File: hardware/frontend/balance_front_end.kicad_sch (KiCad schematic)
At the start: 5 parts, among them Q601 BSS308PE

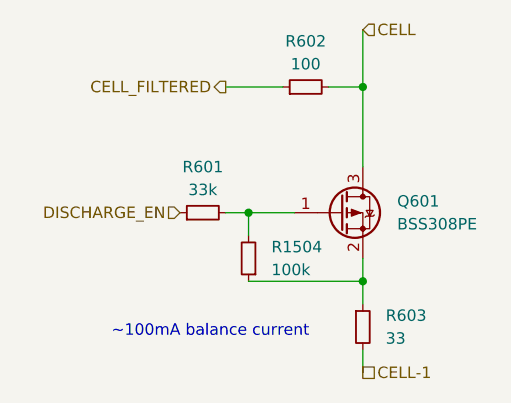
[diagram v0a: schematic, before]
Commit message: footprints assigned
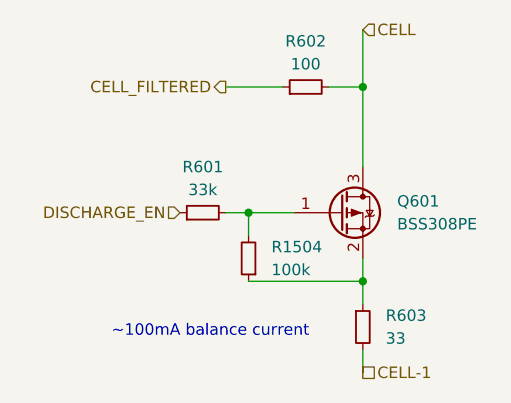
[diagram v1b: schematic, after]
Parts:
- R603: footprint (none) -> Resistor_SMD:R_2512_6332Metric
